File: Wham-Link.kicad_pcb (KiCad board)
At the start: 2 copper layers, 65 x 30 mm, 46 parts, among them J1 Conn_02x08_Counter_Clockwise, SW2 SKRPACE010, SW3 SKRPACE010, U1 LAN8720A-CP-TR, U2 AMS1117-3.3, U3 CH340C, U4 ESP32-WROOM-32UE, X1 ECS-2520MV-250-CN-TR

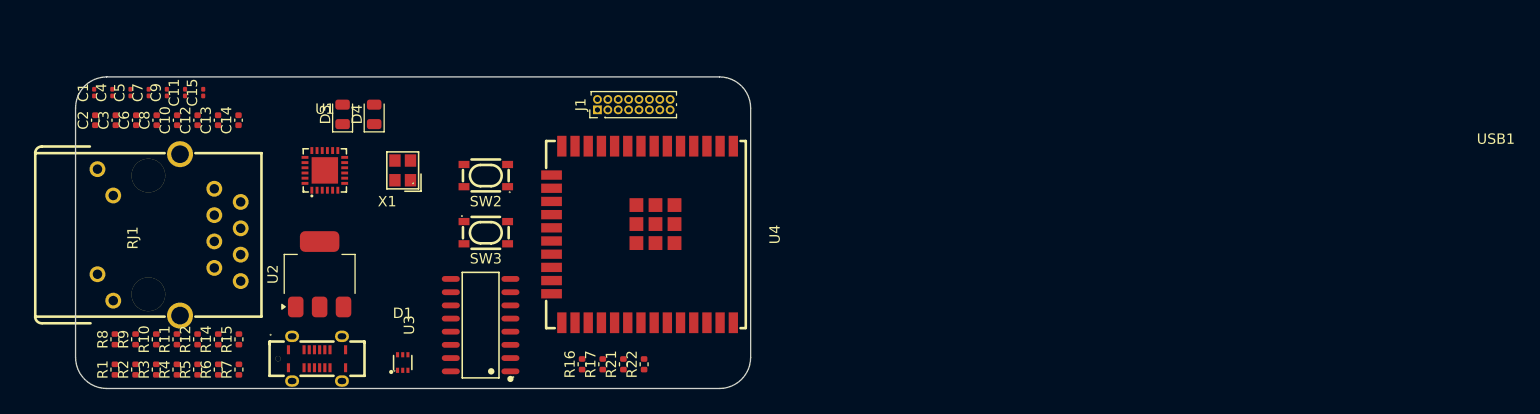
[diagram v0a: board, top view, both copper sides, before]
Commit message: Schematic and library updates
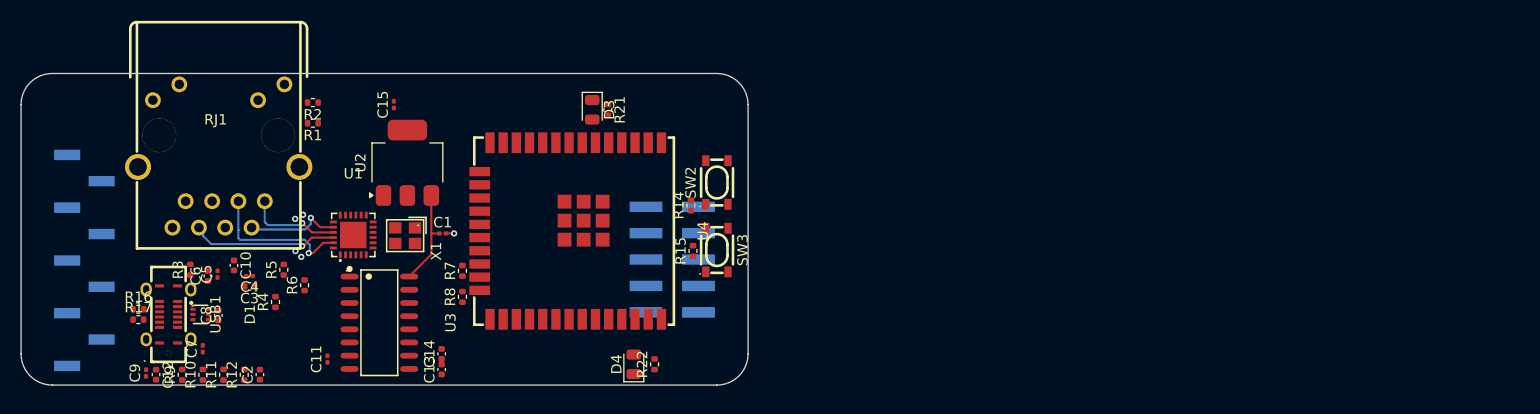
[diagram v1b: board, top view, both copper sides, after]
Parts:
- removed J1: Conn_02x08_Counter_Clockwise, Connector_PinHeader_1.00mm:PinHeader_2x08_P1.00mm_Vertical
- added J2: Conn_02x05_Counter_Clockwise, Connector_PinHeader_2.54mm:PinHeader_2x05_P2.54mm_Vertical_SMD, B.Cu at (175.7, 102.9)
- added J3: Conn_01x09_Pin, Connector_PinHeader_2.54mm:PinHeader_1x09_P2.54mm_Vertical_SMD_Pin1Left, B.Cu at (119.1, 103.0)
- moved R14 47.3 mm to (177.5, 97.7)
- moved R17 44.9 mm to (124.3, 108.7), turned to 0 degrees
- moved R15 44.5 mm to (177.7, 102.1)
- moved R16 43.0 mm to (124.3, 107.7), turned to 0 degrees
- moved C1 36.2 mm to (153.6, 100.4), turned to 0 degrees
- moved D4 34.7 mm to (172.0, 113.0)
- moved R8 33.7 mm to (155.5, 106.5)
- moved C13 32.2 mm to (153.5, 113.5)
- moved R2 30.9 mm to (141.1, 87.8), turned to 180 degrees
- moved R1 30.4 mm to (141.1, 89.8), turned to 180 degrees
- moved C14 29.8 mm to (153.5, 112.0)
- moved C2 29.2 mm to (136.0, 114.0)
- moved C11 29.1 mm to (142.5, 112.5)
- moved C9 27.1 mm to (125.0, 113.8)
- moved C7 25.2 mm to (130.5, 111.5)
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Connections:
- net CLKIN renamed /CLKIN
- net Net-(U1-RXN) renamed /RX-
- net Net-(U1-RXP) renamed /RX+
- net Net-(U1-TXN) renamed /TX-
- net Net-(U1-TXP) renamed /TX+
- C10 pad 1: VDDA -> +3V3
- R10 pad 2: VDDA -> +3V3
- R11 pad 2: VDDA -> +3V3
- R12 pad 2: VDDA -> +3V3
- R9 pad 2: VDDA -> +3V3
- RJ1 pad 4: VDDA -> +3V3
- RJ1 pad 5: VDDA -> +3V3
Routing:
- net /RX-: track 0.00 -> 14.4 mm, vias 0 -> 1
- net /RX+: track 0.00 -> 14.3 mm, vias 0 -> 1
- net /TX+: track 0.00 -> 9.62 mm, vias 0 -> 1
- net +5V: track 0.00 -> 9.46 mm
- net /TX-: track 0.00 -> 9.14 mm, vias 0 -> 1
- net GND: track 0.00 -> 0.78 mm, vias 0 -> 5
- added copper zone on In1.Cu, net GND
- added copper zone on In2.Cu, net GND
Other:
- board size 65 x 30 mm -> 70 x 30 mm
- copper layers 2 -> 4
